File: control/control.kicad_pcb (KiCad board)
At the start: 4 copper layers, 45.7 x 39.4 mm, 90 parts, among them M1 LMR62014, M2 LM46001, M3 STM32F4XX, M4 TPS736XX, M5 SN65HVD23X, P1 GND/VDD, P2 VOLTAGE, P3 INTERFACE, P4 POWER/FETS, P5 SENSOR_A, P6 SENSOR_B, P7 CAN, P8 ANALOG, U1 AD8539

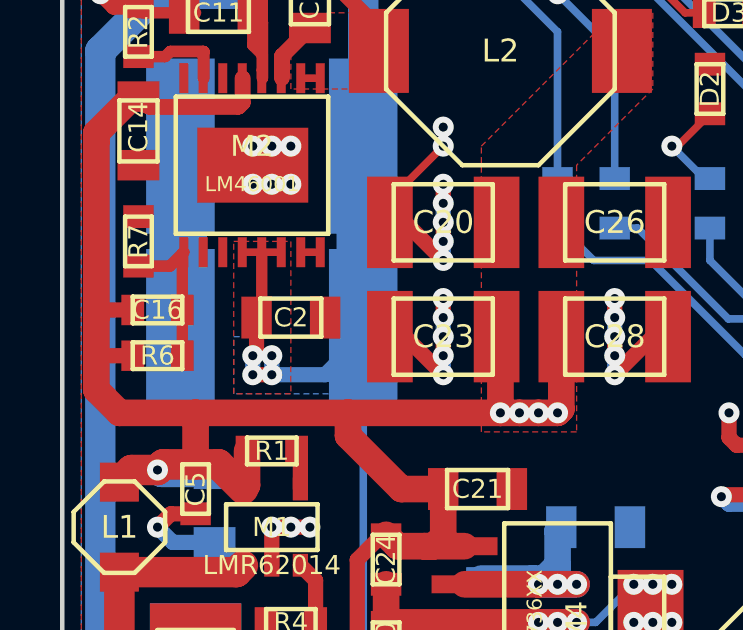
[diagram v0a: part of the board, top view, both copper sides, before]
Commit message: Small fixes for rev2.
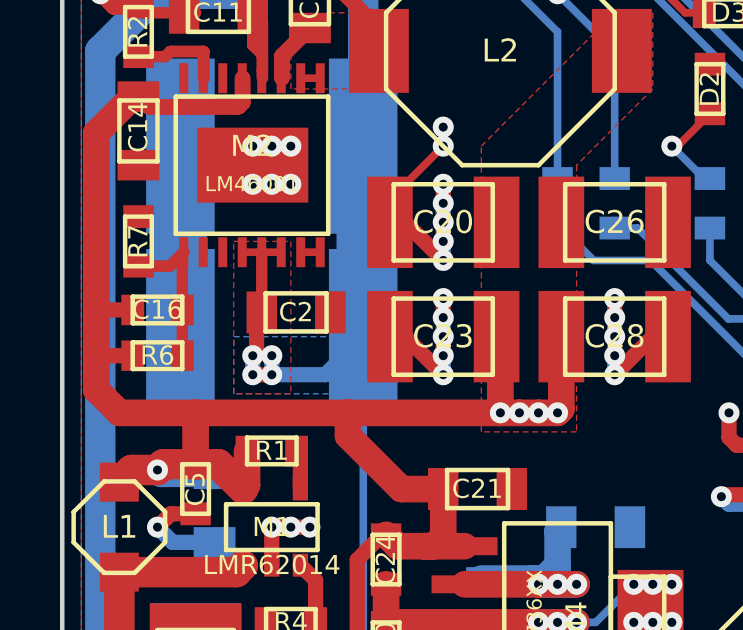
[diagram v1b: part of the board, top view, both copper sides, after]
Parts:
- moved C2 0.24 mm to (104.9, 77.9)
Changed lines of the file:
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@@
     (links 215)
     (no_connects 0)
-    (area 97.079999 60.249999 142.950001 99.770001)
+    (area 96.4311 52.395 155.955 99.770001)
     (thickness 1.6)
     (drawings 6)
@@
   (title_block
     (title "Phobia Control Board")
-    (date 2016-03-31)
+    (date 2016-09-21)
     (rev 2)
     (company "Roman Belov")
@@
   )
   (setup
-    (last_trace_width 0.508)
+    (last_trace_width 0.254)
     (user_trace_width 0.381)
     (user_trace_width 0.508)
@@
       (psnegative false)
       (psa4output false)
-      (plotreference true)
-      (plotvalue true)
+      (plotreference false)
+      (plotvalue false)
       (plotinvisibletext false)
       (padsonsilk false)
@@
   )
   (module foot:SM0805 (layer F.Cu)
-    (at 104.775 78.105)
+    (at 104.948 77.932)
     (attr smd)
     (fp_text reference C2 (at 0 0) (layer F.SilkS)

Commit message: Fixed a few small mistakes.
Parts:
- C6: value 100nF -> 10nF
- C8: value 10nF -> 100nF
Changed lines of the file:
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@@
-(kicad_pcb (version 4) (host pcbnew 4.0.2-stable)
+(kicad_pcb (version 4) (host pcbnew 4.0.4-stable)
   (general
     (links 215)
     (no_connects 0)
-    (area 96.4311 52.395 155.955 99.770001)
+    (area 97.079999 60.249999 142.950001 99.770001)
     (thickness 1.6)
     (drawings 6)
@@
       (effects (font (size 0.635 0.635) (thickness 0.127)))
     )
-    (fp_text value 100nF (at 0 -1.397 180) (layer F.SilkS) hide
+    (fp_text value 10nF (at 0 -1.397 180) (layer F.SilkS) hide
       (effects (font (size 0.635 0.635) (thickness 0.127)))
     )
@@
       (effects (font (size 0.635 0.635) (thickness 0.127)))
     )
-    (fp_text value 10nF (at 0 -1.397 270) (layer F.SilkS) hide
+    (fp_text value 100nF (at 0 -1.397 270) (layer F.SilkS) hide
       (effects (font (size 0.635 0.635) (thickness 0.127)))
     )
@@
         (xy 135.89 85.09) (xy 135.89 93.345) (xy 142.24 93.345) (xy 142.24 99.06) (xy 104.14 99.06)
         (xy 104.14 95.25) (xy 106.68 92.71) (xy 129.54 92.71) (xy 130.81 91.44) (xy 130.81 88.9)
-        (xy 128.905 86.995) (xy 128.905 83.058) (xy 133.858 83.058) (xy 135.89 85.09)
+        (xy 128.905 86.995) (xy 128.905 83.058) (xy 133.858 83.058)
       )
     )
@@
         (xy 135.89 85.09) (xy 135.89 93.345) (xy 142.24 93.345) (xy 142.24 99.06) (xy 104.14 99.06)
         (xy 104.14 95.25) (xy 106.68 92.71) (xy 129.54 92.71) (xy 130.81 91.44) (xy 130.81 88.9)
-        (xy 128.905 86.995) (xy 128.905 83.058) (xy 133.858 83.058) (xy 135.89 85.09)
+        (xy 128.905 86.995) (xy 128.905 83.058) (xy 133.858 83.058)
       )
     )
